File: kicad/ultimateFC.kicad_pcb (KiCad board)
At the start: 8 copper layers, 30.4 x 25.2 mm, 192 parts, among them J1 USB_B_Micro, J2 10132797-011100LF, J3 10132797-011100LF, J4 10132797-011100LF, J5 10132797-011100LF, J6 10132797-011100LF, Q1 DMP2066LSN-7, U1 EFM8BB21F16G-C-QFN20R, U10 NCP81253MNTBG, U11 SiZ200DT, U12 NCP81253MNTBG, U13 SiZ200DT, U14 TPS62821, U15 SiZ200DT, U16 NCP81253MNTBG, U17 NCP81253MNTBG, U18 NCP81253MNTBG, U19 NCP81253MNTBG, U2 EFM8BB21F16G-C-QFN20R, U20 SiZ200DT, U21 SiZ200DT, U22 SiZ200DT, U23 SiZ200DT, U24 EFM8BB21F16G-C-QFN20R, U25 NCP81253MNTBG, U26 SiZ200DT, U27 NCP81253MNTBG, U28 NCP81253MNTBG, U29 SiZ200DT, U3 NCP81253MNTBG, U30 SiZ200DT, U31 INA186, U32 LMR33630CQRNX, U33 STM32F745VGHx, U34 AB7456, U35 ZOE-M8Q_ZOE-M8Q, U36 ICM-20602, U37 S25FL064L, U39 BMP280, U4 SiZ200DT, U6 EFM8BB21F16G-C-QFN20R, U7 NCP81253MNTBG, U8 SiZ200DT, U9 NCP81253MNTBG, X1 Molex_734120110, Y1 CSTNE8M00G550000R0, Y2 ECS-270-8-47Q-CES-TR

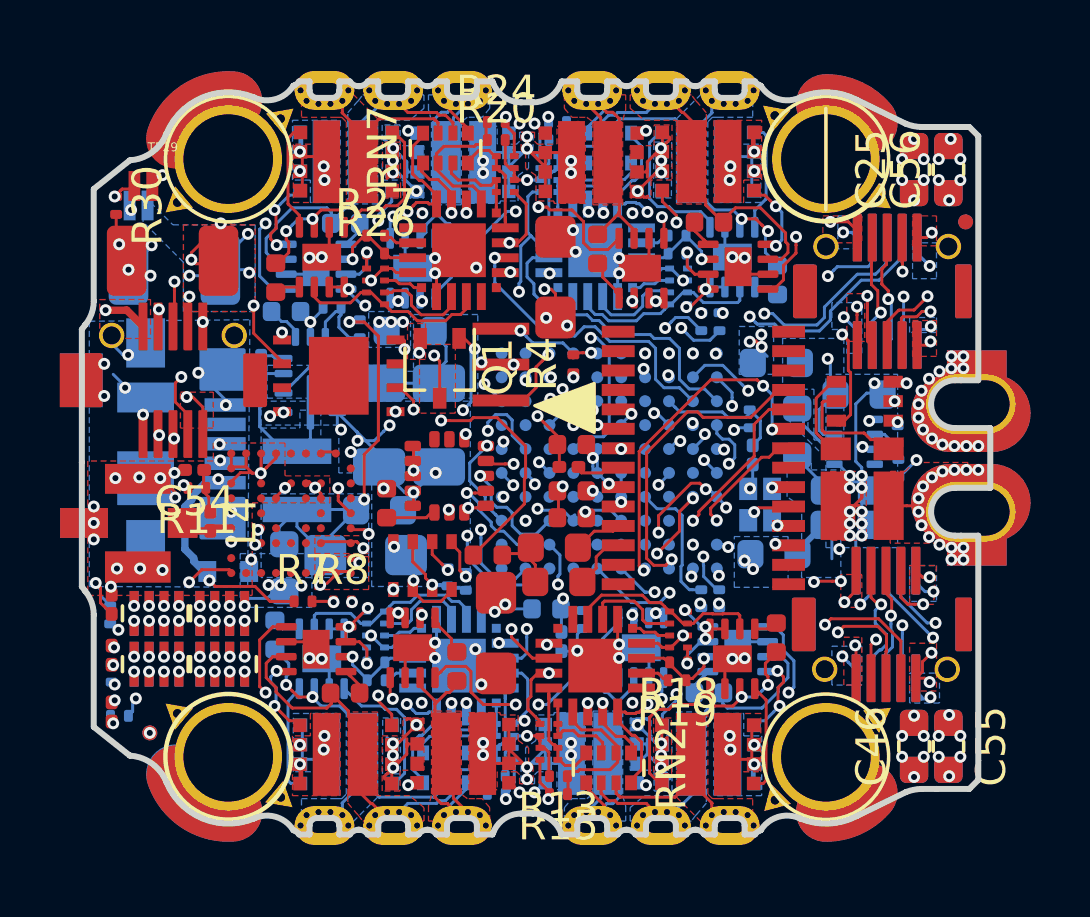
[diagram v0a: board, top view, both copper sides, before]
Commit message: Cleaned up a bit
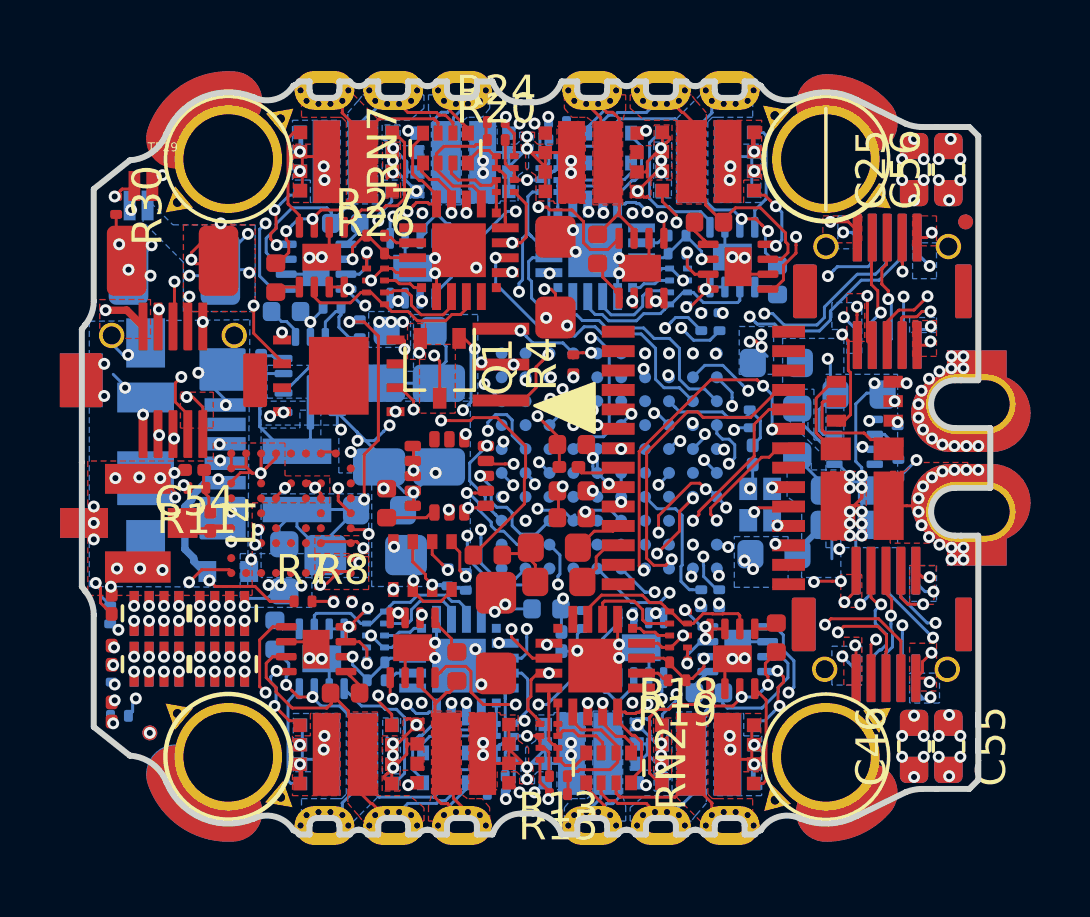
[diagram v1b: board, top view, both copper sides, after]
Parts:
- removed the REF** at (197.1, 64.1) (x2)
- added REF**: Fiducial_0.5mm_Dia_1mm_Outer, Fiducial:Fiducial_0.5mm_Dia_1mm_Outer, F.Cu at (197.1, 64.1)
- added REF**: Fiducial_0.5mm_Dia_1mm_Outer, Fiducial:Fiducial_0.5mm_Dia_1mm_Outer, B.Cu at (197.1, 64.1)

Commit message: added images
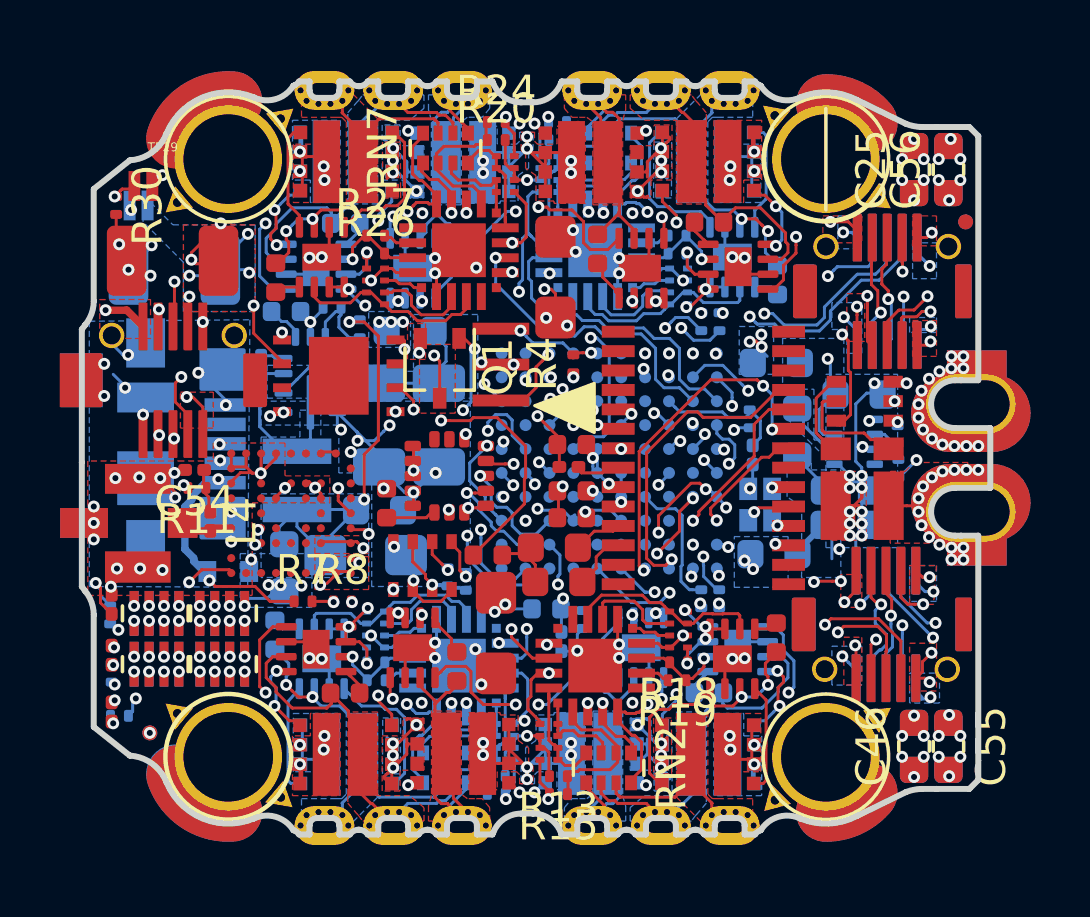
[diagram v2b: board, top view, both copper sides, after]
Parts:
- removed the REF** at (197.1, 64.1) (x2)
- added REF**: Fiducial_0.5mm_Dia_1mm_Outer, Fiducial:Fiducial_0.5mm_Dia_1mm_Outer, F.Cu at (197.1, 64.1)
- added REF**: Fiducial_0.5mm_Dia_1mm_Outer, Fiducial:Fiducial_0.5mm_Dia_1mm_Outer, B.Cu at (197.1, 64.1)
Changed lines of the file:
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@@
     (polygon
       (pts
-        (xy 174.9 70.4) (xy 175.6 70.4) (xy 175.6 71.8) (xy 173.6 71.8) (xy 173.6 71)
-        (xy 174.9 71)
+        (xy 174.9 70.4) (xy 175.6 70.4) (xy 175.6 71.8) (xy 173.6 71.8) (xy 173.6 71.3)
+        (xy 174.9 71.3)
       )
     )
